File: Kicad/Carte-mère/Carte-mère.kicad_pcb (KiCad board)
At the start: 2 copper layers, 21 parts, among them P1 CONN_01X10, P2 CONN_01X04, P3 CONN_01X06, P4 CONN_01X06, P5 CONN_01X04, P6 CONN_01X04, P7 CONN_01X02

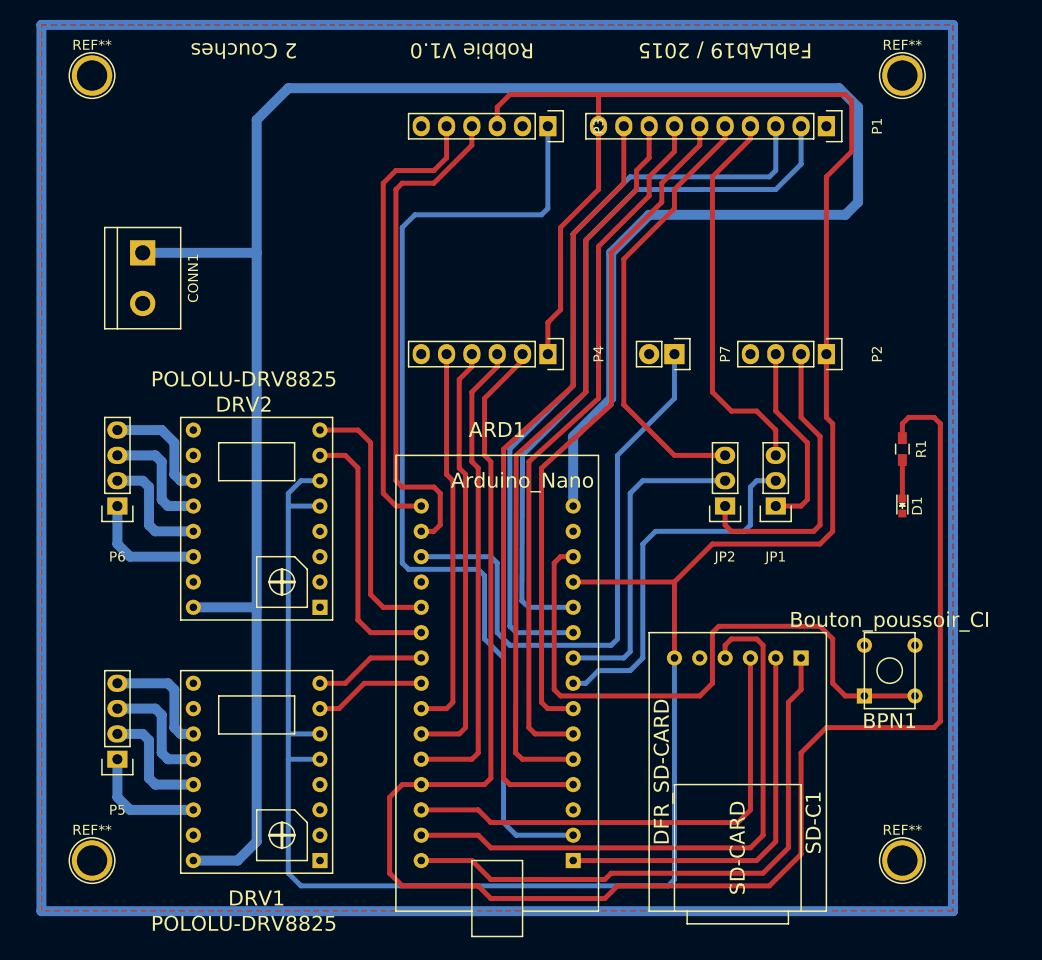
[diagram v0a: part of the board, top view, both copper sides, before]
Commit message: Ajout de la refonte de la carte mère
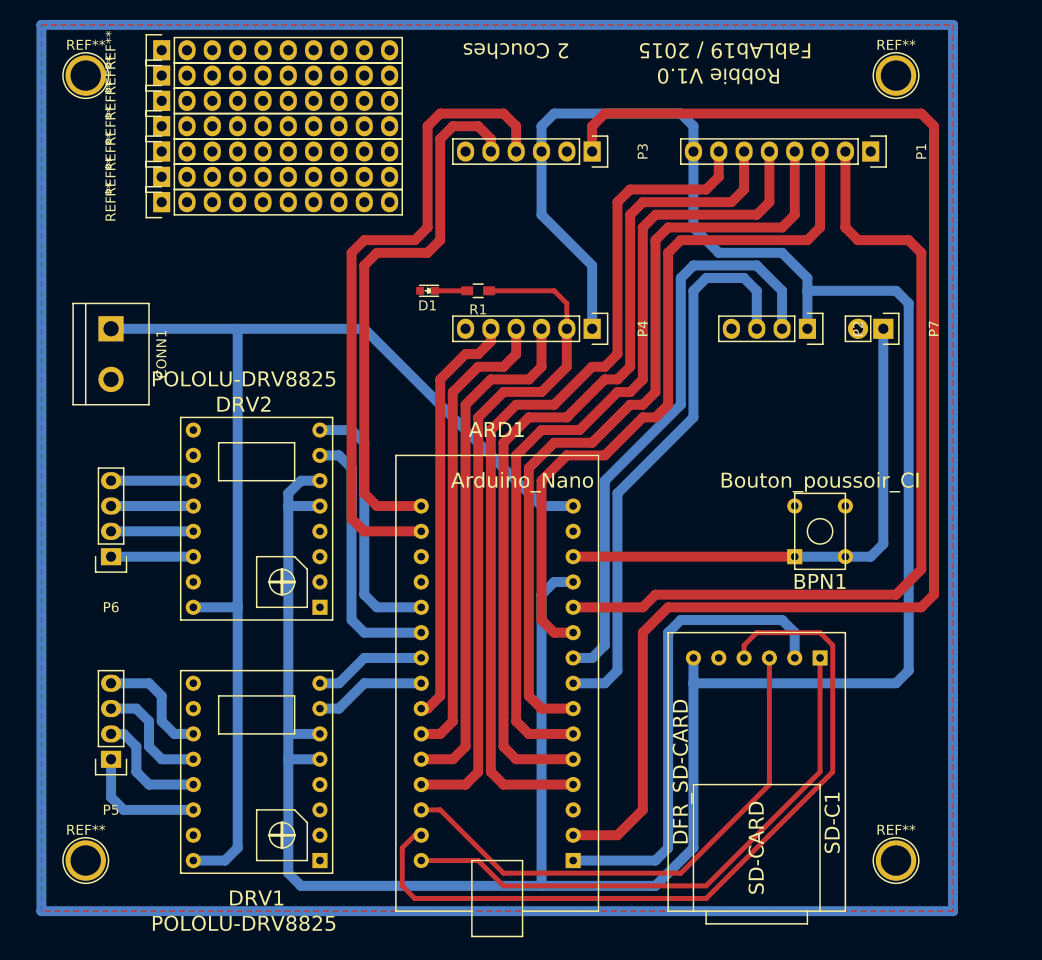
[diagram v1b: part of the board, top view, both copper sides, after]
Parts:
- removed JP1, JP2: JUMPER3, Pin_Headers:Pin_Header_Straight_1x03
- removed the REF** at (191.1, 147.3)
- removed the REF** at (109.9, 147.3)
- removed the REF** at (109.9, 68.6)
- removed the REF** at (191.1, 68.6)
- added REF**: 1pin, Connect:1pin, F.Cu at (109.2, 68.6)
- added REF**: Pin_Header_Straight_1x10, Pin_Headers:Pin_Header_Straight_1x10, F.Cu at (116.8, 78.7)
- added REF**: Pin_Header_Straight_1x10, Pin_Headers:Pin_Header_Straight_1x10, F.Cu at (116.8, 81.3)
- added REF**: 1pin, Connect:1pin, F.Cu at (190.5, 68.6)
- added REF**: 1pin, Connect:1pin, F.Cu at (190.5, 147.3)
- added REF**: 1pin, Connect:1pin, F.Cu at (109.2, 147.3)
- added REF**: Pin_Header_Straight_1x10, Pin_Headers:Pin_Header_Straight_1x10, F.Cu at (116.8, 66.0)
- added REF**: Pin_Header_Straight_1x10, Pin_Headers:Pin_Header_Straight_1x10, F.Cu at (116.8, 68.6)
- added REF**: Pin_Header_Straight_1x10, Pin_Headers:Pin_Header_Straight_1x10, F.Cu at (116.8, 71.1)
- added REF**: Pin_Header_Straight_1x10, Pin_Headers:Pin_Header_Straight_1x10, F.Cu at (116.8, 73.7)
- added REF**: Pin_Header_Straight_1x10, Pin_Headers:Pin_Header_Straight_1x10, F.Cu at (116.8, 76.2)
- P1: value CONN_01X10 -> CONN_01X08; footprint Pin_Headers:Pin_Header_Straight_1x10 -> Pin_Headers:Pin_Header_Straight_1x08
- moved D1 52.3 mm to (143.5, 90.2), turned to 180 degrees
- moved R1 45.4 mm to (148.6, 90.2), turned to 180 degrees
- moved P7 21.1 mm to (189.2, 94.0)
- moved BPN1 15.6 mm to (182.9, 114.3)
- moved CONN1 8.25 mm to (111.8, 96.5)
- moved P1 5.12 mm to (188.0, 76.2)
- moved P3 5.12 mm to (160.0, 76.2)
- moved P4 5.12 mm to (160.0, 94.0)
- moved P6 5.12 mm to (111.8, 116.8)
- moved P2 3.17 mm to (181.6, 94.0)
- moved SD-C1 1.91 mm to (175.3, 127.0)
- moved P5 0.63 mm to (111.8, 137.2)
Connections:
- ARD1 pad 18: Net-(ARD1-Pad18) -> (no net)
- P1 pad 4: Net-(JP1-Pad3) -> Net-(ARD1-Pad7)
- P1 pad 5: Net-(JP2-Pad3) -> Net-(ARD1-Pad6)
- P1 pad 6: Net-(ARD1-Pad7) -> Net-(ARD1-Pad5)
- P1 pad 7: Net-(ARD1-Pad6) -> Net-(ARD1-Pad4)
- P1 pad 8: Net-(ARD1-Pad5) -> +5V
- P2 pad 2: Net-(JP2-Pad1) -> Net-(ARD1-Pad9)
- P2 pad 3: Net-(JP1-Pad1) -> Net-(ARD1-Pad8)
- P3 pad 2: (no net) -> GND
- P7 pad 1: Net-(ARD1-Pad18) -> Net-(ARD1-Pad13)
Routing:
- net +BATT: track 223.1 -> 115.2 mm
- net Net-(ARD1-Pad27): track 168.2 -> 67.5 mm
- net Net-(ARD1-Pad18): track 58.7 -> 0.00 mm
- net Net-(JP2-Pad3): track 44.4 -> 0.00 mm
- net +3.3V: track 99.2 -> 141.5 mm
- net Net-(JP1-Pad3): track 38.7 -> 0.00 mm
- net Net-(JP2-Pad1): track 29.9 -> 0.00 mm
- net Net-(ARD1-Pad9): track 31.9 -> 59.2 mm
- net +5V: track 259.7 -> 283.2 mm
- net Net-(ARD1-Pad8): track 37.7 -> 57.5 mm
- net Net-(JP1-Pad1): track 19.4 -> 0.00 mm
- net Net-(ARD1-Pad29): track 60.0 -> 79.1 mm
- net Net-(ARD1-Pad17): track 50.9 -> 65.5 mm
- net Net-(ARD1-Pad7): track 68.0 -> 80.3 mm
- net Net-(ARD1-Pad11): track 72.8 -> 84.5 mm
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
